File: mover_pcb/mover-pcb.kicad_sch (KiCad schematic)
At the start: 9 parts, among them J1 Conn_01x03_Pin, J2 Conn_01x05_Pin, J3 Conn_01x05_Pin, J4 Conn_01x06_Pin, J5 Conn_01x04_Pin, J6 Conn_01x03_Pin

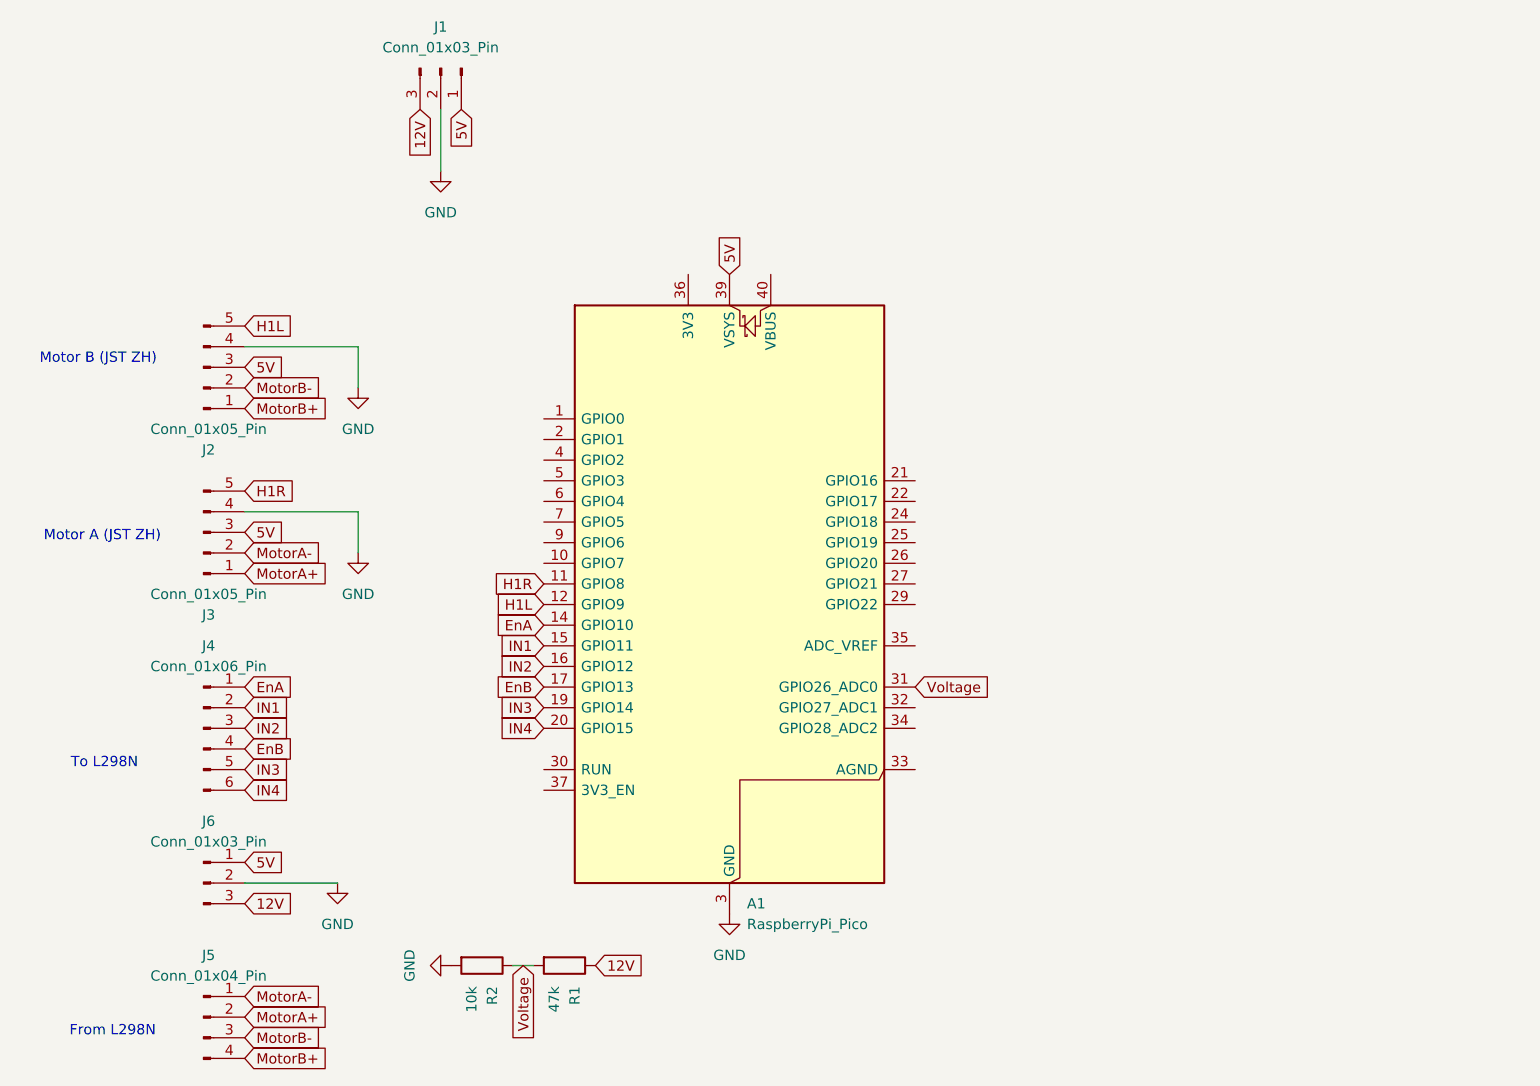
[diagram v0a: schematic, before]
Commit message: update pcb; progress on controller
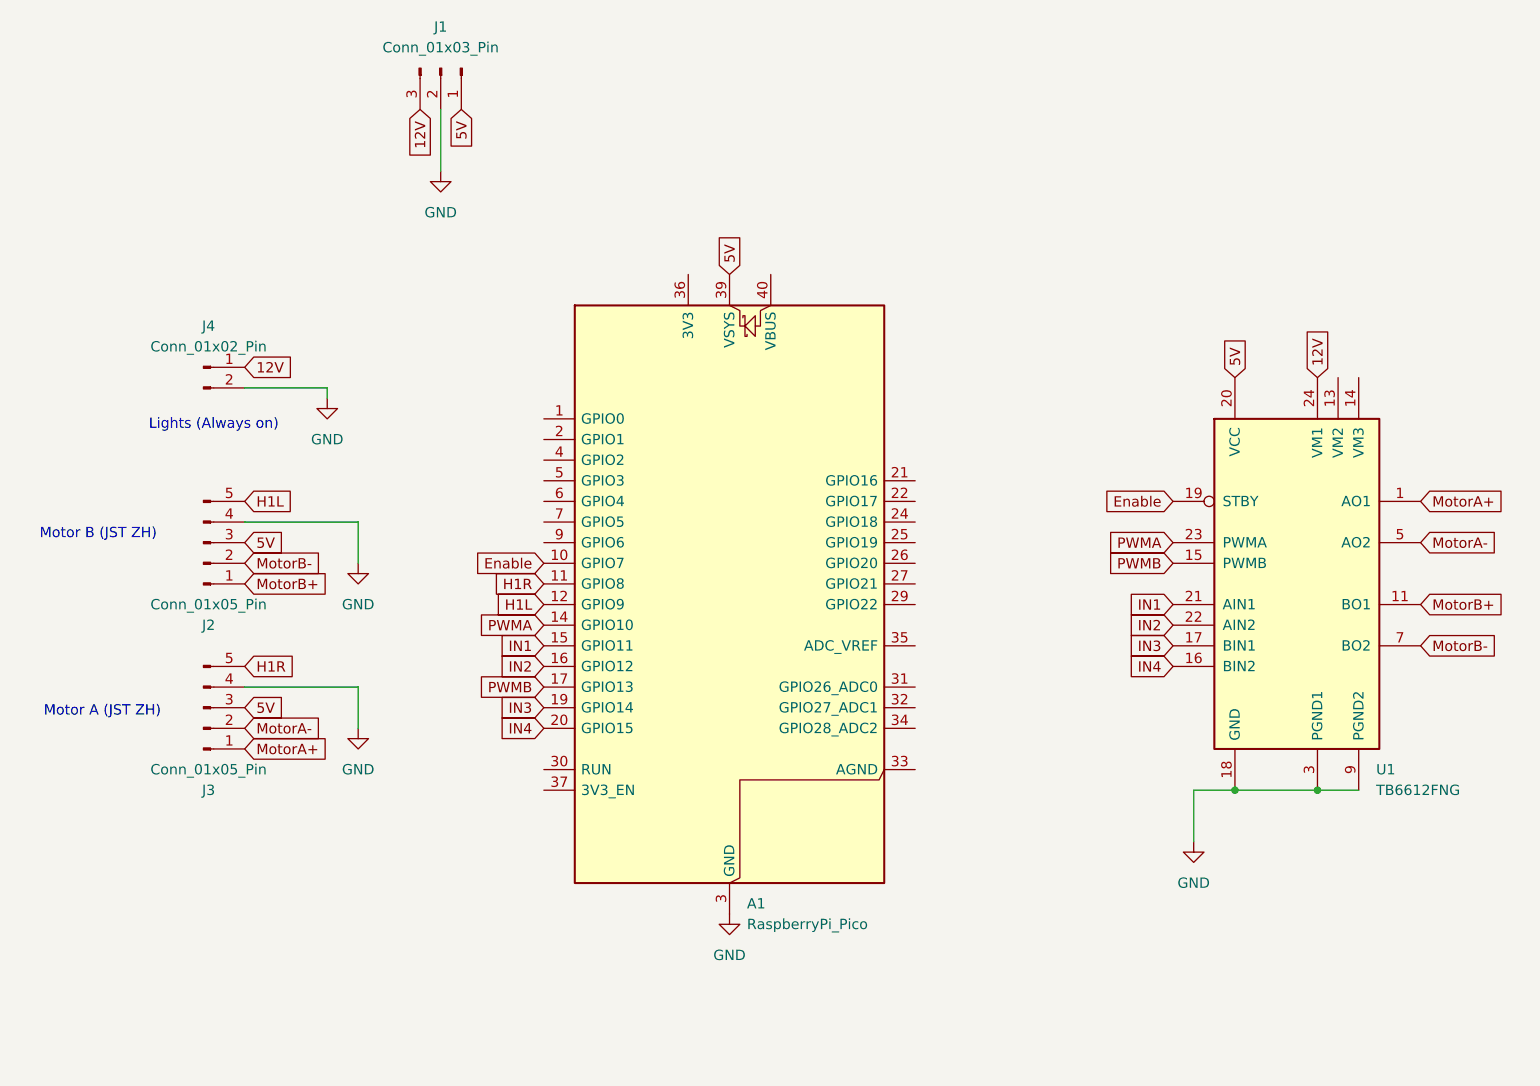
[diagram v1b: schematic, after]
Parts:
- removed J4: Conn_01x06_Pin, Connector_PinHeader_2.54mm:PinHeader_1x06_P2.54mm_Vertical, symbol Connector:Conn_01x06_Pin
- removed J5: Conn_01x04_Pin, TerminalBlock_Phoenix:TerminalBlock_Phoenix_MKDS-1,5-4-5.08_1x04_P5.08mm_Horizontal, symbol Connector:Conn_01x04_Pin
- removed J6: Conn_01x03_Pin, TerminalBlock_Phoenix:TerminalBlock_Phoenix_MKDS-1,5-3-5.08_1x03_P5.08mm_Horizontal, symbol Connector:Conn_01x03_Pin
- removed R1: 47k, Resistor_THT:R_Axial_DIN0207_L6.3mm_D2.5mm_P7.62mm_Horizontal, symbol Device:R
- removed R2: 10k, Resistor_THT:R_Axial_DIN0207_L6.3mm_D2.5mm_P7.62mm_Horizontal, symbol Device:R
- added J4: Conn_01x02_Pin, TerminalBlock_Phoenix:TerminalBlock_Phoenix_MKDS-1,5-2-5.08_1x02_P5.08mm_Horizontal, symbol Connector:Conn_01x02_Pin
- added U1: TB6612FNG, TB6612:TB6612FNG_Module, symbol Driver_Motor:TB6612FNG
- A1: footprint Module:RaspberryPi_Pico_Common_SMD -> Module:RaspberryPi_Pico_Common_THT
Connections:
- net 12V: now also J4.1 (Pin_1), U1.24 (VM1)
- net 5V: now also U1.20 (VCC)
- net GND: now also J4.2 (Pin_2), U1.10 (PGND2), U1.18 (GND), U1.3 (PGND1), U1.4 (PGND1), U1.9 (PGND2)
- net IN1: now also U1.21 (AIN1)
- net IN2: now also U1.22 (AIN2)
- net IN3: now also U1.17 (BIN1)
- net IN4: now also U1.16 (BIN2)
- net MotorA+: now also U1.1 (AO1), U1.2 (AO1)
- net MotorA-: now also U1.5 (AO2), U1.6 (AO2)
- net MotorB+: now also U1.11 (BO1), U1.12 (BO1)
- net MotorB-: now also U1.7 (BO2), U1.8 (BO2)
- net Enable: now reaches A1.10 (GPIO7)
- net Enable: now also U1.19 (STBY)
- net EnA renamed PWMA
- net PWMA: now also U1.23 (PWMA)
- net EnB renamed PWMB
- net PWMB: now also U1.15 (PWMB)
- net Voltage: no longer names the net of A1.31 (GPIO26_ADC0)
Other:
- note added: "Lights (Always on)"
- note removed: "From L298N"
- note removed: "To L298N"
- moved on the sheet: J2, J3
